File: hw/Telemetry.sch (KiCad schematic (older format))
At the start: 37 parts, among them J102 BOOT0, J103 SPORT, J104 SBUS, J105 USB_B_Micro, J106 UART_EXP, SW101 SW_Push, U101 STM32F303CBx, U102 IS25LP032D, X101 SG-310_SCF_8.000000MHZ

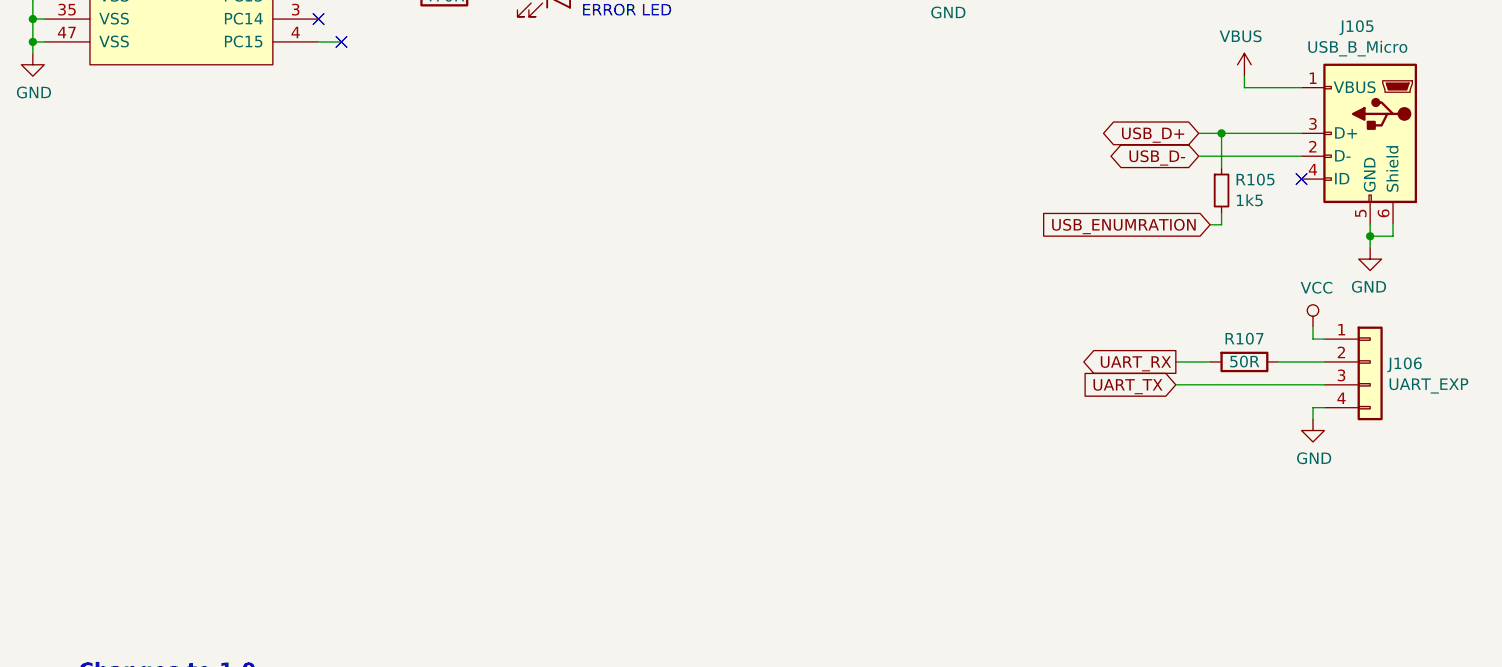
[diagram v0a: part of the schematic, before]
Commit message: Routing update
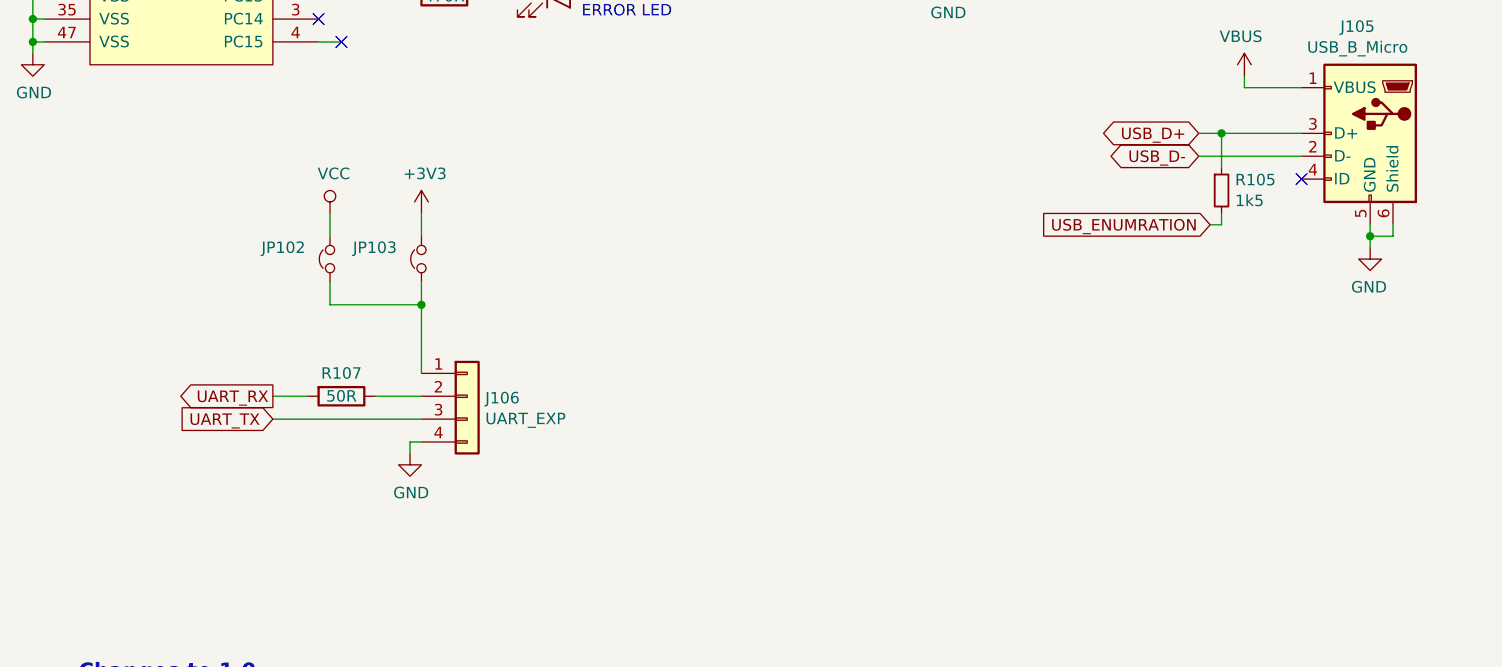
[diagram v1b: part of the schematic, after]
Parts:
- added JP102, JP103: Jumper_NC_Small, Resistor_SMD:R_0402_1005Metric, symbol Device:Jumper_NC_Small
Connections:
- net +3V3: now also JP103.2
- net VCC: now also JP102.2; no longer J106.1 (Pin_1)
- new net: J106.1 (Pin_1), JP102.1, JP103.1
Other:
- moved on the sheet: J106, R107
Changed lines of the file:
@@
 L power:GND #PWR0122
 U 1 1 5CE5F3AC
-P 10400 6250
-F 0 "#PWR0122" H 10400 6000 50  0001 C CNN
-F 1 "GND" H 10405 6077 50  0000 C CNN
-F 2 "" H 10400 6250 50  0001 C CNN
-F 3 "" H 10400 6250 50  0001 C CNN
-	1    10400 6250
-	1    0    0    -1
-$EndComp
-Wire Wire Line
-	10450 6200 10400 6200
-Wire Wire Line
-	10400 6200 10400 6250
-$Comp
-L Connector_Generic:Conn_01x04 J106
-U 1 1 5CE6386B
-P 10650 6000
-F 0 "J106" H 10729 5992 50  0000 L CNN
-F 1 "UART_EXP" H 10729 5901 50  0000 L CNN
-F 2 "Connector_PinHeader_2.54mm:PinHeader_2x02_P2.54mm_Vertical" H 10650 6000 50  0001 C CNN
-F 3 "~" H 10650 6000 50  0001 C CNN
-F 4 "-prod" H 10650 6000 50  0001 C CNN "Config"
-	1    10650 6000
-	1    0    0    -1
-$EndComp
-Wire Wire Line
-	10450 5900 10400 5900
-Wire Wire Line
-	10400 5900 10400 5850
-$Comp
-L power:VCC #PWR0123
-U 1 1 5CE67EB7
-P 10400 5850
-F 0 "#PWR0123" H 10400 5700 50  0001 C CNN
-F 1 "VCC" H 10417 6023 50  0000 C CNN
-F 2 "" H 10400 5850 50  0001 C CNN
-F 3 "" H 10400 5850 50  0001 C CNN
-	1    10400 5850
-	1    0    0    -1
-$EndComp
+P 6450 6400
+F 0 "#PWR0122" H 6450 6150 50  0001 C CNN
+F 1 "GND" H 6455 6227 50  0000 C CNN
+F 2 "" H 6450 6400 50  0001 C CNN
+F 3 "" H 6450 6400 50  0001 C CNN
+	1    6450 6400
+	1    0    0    -1
+$EndComp
+Wire Wire Line
+	6500 6350 6450 6350
+Wire Wire Line
+	6450 6350 6450 6400
 Text GLabel 6150 3900 2    50   Input ~ 0
 BAT_VOLTAGE
@@
 	1    0    0    -1
 $EndComp
-Text GLabel 9800 6000 0    50   Output ~ 0
+Text GLabel 5850 6150 0    50   Output ~ 0
 UART_RX
-Text GLabel 9800 6100 0    50   Input ~ 0
+Text GLabel 5850 6250 0    50   Input ~ 0
 UART_TX
 Text GLabel 6150 3100 2    50   Output ~ 0
@@
 L Device:R R107
 U 1 1 5E51659E
-P 10100 6000
-F 0 "R107" V 10000 6000 50  0000 C CNN
-F 1 "50R" V 10100 6000 50  0000 C CNN
-F 2 "Resistor_SMD:R_0603_1608Metric_Pad1.05x0.95mm_HandSolder" V 10030 6000 50  0001 C CNN
-F 3 "~" H 10100 6000 50  0001 C CNN
-	1    10100 6000
+P 6150 6150
+F 0 "R107" V 6050 6150 50  0000 C CNN
+F 1 "50R" V 6150 6150 50  0000 C CNN
+F 2 "Resistor_SMD:R_0603_1608Metric_Pad1.05x0.95mm_HandSolder" V 6080 6150 50  0001 C CNN
+F 3 "~" H 6150 6150 50  0001 C CNN
+	1    6150 6150
 	0    1    1    0
 $EndComp
 Wire Wire Line
-	9950 6000 9800 6000
-Wire Wire Line
-	10250 6000 10450 6000
+	6000 6150 5850 6150
+Wire Wire Line
+	6300 6150 6500 6150
 $Comp
 L Device:R R108
@@
 	6050 3000 6500 3000
 Wire Wire Line
-	9800 6100 10450 6100
+	5850 6250 6500 6250
 Wire Wire Line
 	4800 4050 4800 4400
@@
 $EndComp
 NoConn ~ 6150 4600
+$Comp
+L power:VCC #PWR0123
+U 1 1 5CE67EB7
+P 6100 5350
+F 0 "#PWR0123" H 6100 5200 50  0001 C CNN
+F 1 "VCC" H 6117 5523 50  0000 C CNN
+F 2 "" H 6100 5350 50  0001 C CNN
+F 3 "" H 6100 5350 50  0001 C CNN
+	1    6100 5350
+	1    0    0    -1
+$EndComp
+$Comp
+L power:+3V3 #PWR0144
+U 1 1 5E59175F
+P 6500 5350
+F 0 "#PWR0144" H 6500 5200 50  0001 C CNN
+F 1 "+3V3" H 6515 5523 50  0000 C CNN
+F 2 "" H 6500 5350 50  0001 C CNN
+F 3 "" H 6500 5350 50  0001 C CNN
+	1    6500 5350
+	1    0    0    -1
+$EndComp
+Wire Wire Line
+	6100 5750 6100 5650
+Wire Wire Line
+	6100 5750 6500 5750
+Wire Wire Line
+	6100 5450 6100 5350
+Wire Wire Line
+	6500 5350 6500 5450
+Wire Wire Line
+	6500 5650 6500 5750
+$Comp
+L Connector_Generic:Conn_01x04 J106
+U 1 1 5CE6386B
+P 6700 6150
+F 0 "J106" H 6779 6142 50  0000 L CNN
+F 1 "UART_EXP" H 6779 6051 50  0000 L CNN
+F 2 "Connector_PinHeader_2.54mm:PinHeader_2x02_P2.54mm_Vertical" H 6700 6150 50  0001 C CNN
+F 3 "~" H 6700 6150 50  0001 C CNN
+F 4 "-prod" H 6700 6150 50  0001 C CNN "Config"
+	1    6700 6150
+	1    0    0    -1
+$EndComp
+Connection ~ 6500 5750
+$Comp
+L Device:Jumper_NC_Small JP103
+U 1 1 5E5F175F
+P 6500 5550
+F 0 "JP103" V 6550 5850 50  0000 R CNN
+F 1 "Jumper_NC_Small" V 6455 5503 50  0001 R CNN
+F 2 "Resistor_SMD:R_0402_1005Metric" H 6500 5550 50  0001 C CNN
+F 3 "~" H 6500 5550 50  0001 C CNN
+F 4 "dnp" H 6500 5550 50  0001 C CNN "Config"
+	1    6500 5550
+	0    -1   -1   0
+$EndComp
+$Comp
+L Device:Jumper_NC_Small JP102
+U 1 1 5E5F3931
+P 6100 5550
+F 0 "JP102" V 6150 5850 50  0000 R CNN
+F 1 "Jumper_NC_Small" V 6050 6300 50  0001 R CNN
+F 2 "Resistor_SMD:R_0402_1005Metric" H 6100 5550 50  0001 C CNN
+F 3 "~" H 6100 5550 50  0001 C CNN
+F 4 "dnp" H 6100 5550 50  0001 C CNN "Config"
+	1    6100 5550
+	0    -1   -1   0
+$EndComp
+Wire Wire Line
+	6500 5750 6500 6050
 $EndSCHEMATC
